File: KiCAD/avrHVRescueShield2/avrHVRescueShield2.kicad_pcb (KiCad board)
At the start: 2 copper layers, 69.8 x 54.6 mm, 24 parts, among them Q1 MUN5311DW1T1G, SW1 SW_Push, U1 ATmega328P-PU, U2 ATtiny85-20PU, U3 ATtiny2313-20PU, U4 MC34063AP

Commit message: error in schematics
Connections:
- U1 pad 1: unconnected-(U1-Pad1) -> ~{RESET}
- U1 pad 21: ~{RESET} -> unconnected-(U1-Pad21)
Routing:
- net GND: track 203.6 -> 390.5 mm
- net ~{RESET}: track 93.3 -> 0.00 mm
- net RDY: track 54.4 -> 0.00 mm
- net DATA6: track 39.2 -> 0.00 mm

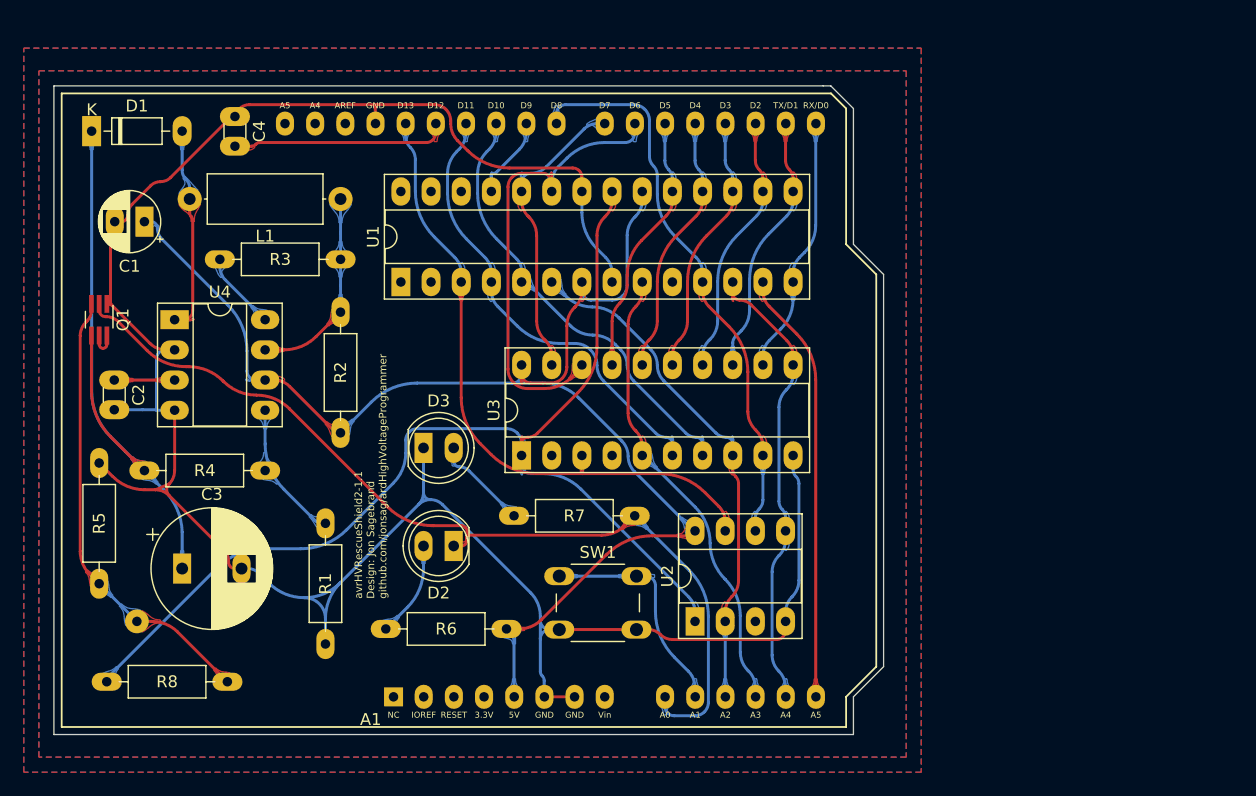
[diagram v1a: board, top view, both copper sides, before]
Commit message: new PCB
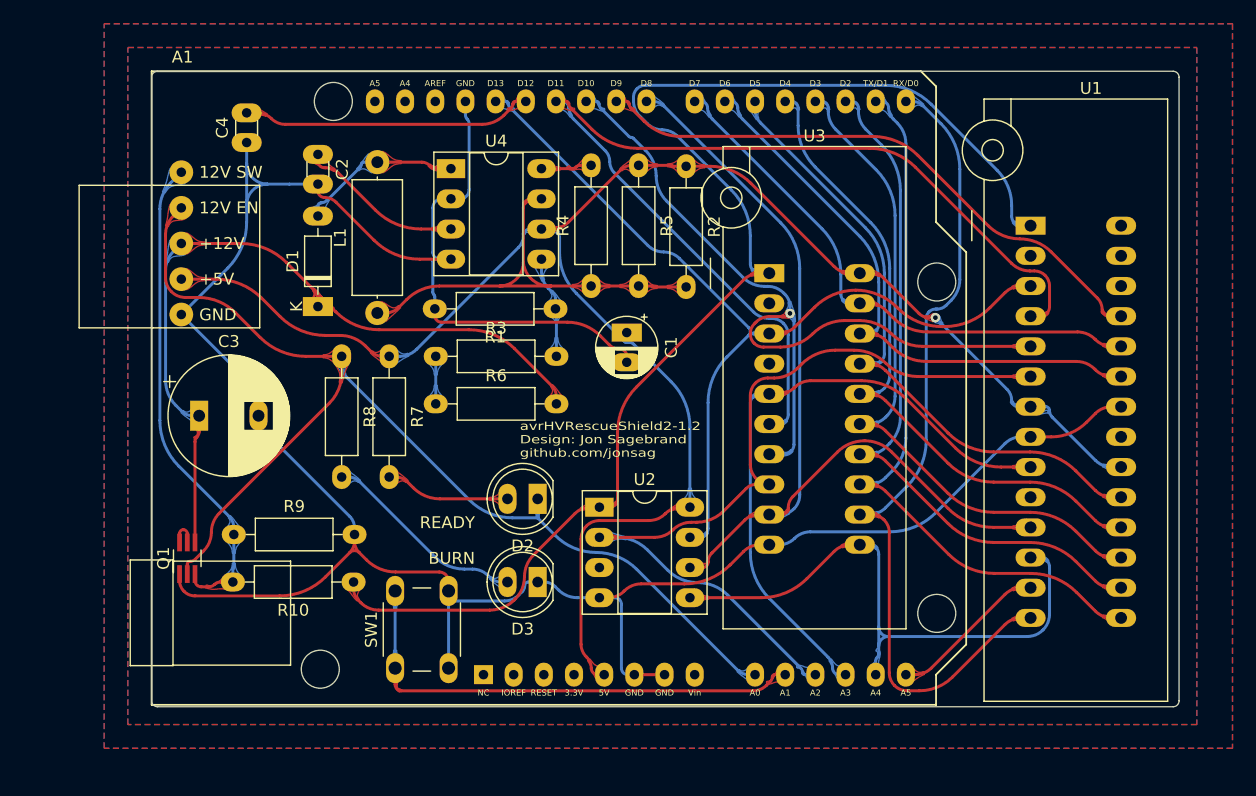
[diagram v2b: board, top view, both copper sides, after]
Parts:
- added R10: 100R, My_Misc:R_Axial_DIN0207_L6.3mm_D2.5mm_P10.16mm_Horizontal_large, F.Cu at (130.0, 104.0)
- added R9: 1k, My_Misc:R_Axial_DIN0207_L6.3mm_D2.5mm_P10.16mm_Horizontal_large, F.Cu at (119.9, 100.0)
- added TP2: 12V EN, My_Misc:Single_solder_pad, F.Cu at (115.5, 72.5)
- added TP3: 12V SW, My_Misc:Single_solder_pad, F.Cu at (115.5, 69.5)
- added TP4: +5V, My_Misc:Single_solder_pad, F.Cu at (115.5, 78.5)
- added TP5: GND, My_Misc:Single_solder_pad, F.Cu at (115.5, 81.5)
- R1, R7: footprint My_Misc:R_Axial_DIN0207_L6.3mm_D2.5mm_P10.16mm_Horizontal_larger_pads -> My_Misc:R_Axial_DIN0207_L6.3mm_D2.5mm_P10.16mm_Horizontal_large
- R2: value 0.5R -> 1R; footprint My_Misc:R_Axial_DIN0207_L6.3mm_D2.5mm_P10.16mm_Horizontal_larger_pads -> My_Misc:R_Axial_DIN0207_L6.3mm_D2.5mm_P10.16mm_Horizontal_large
- R3: value 180R -> 12k; footprint My_Misc:R_Axial_DIN0207_L6.3mm_D2.5mm_P10.16mm_Horizontal_larger_pads -> My_Misc:R_Axial_DIN0207_L6.3mm_D2.5mm_P10.16mm_Horizontal_large
- R4: value 13k -> 180R; footprint My_Misc:R_Axial_DIN0207_L6.3mm_D2.5mm_P10.16mm_Horizontal_larger_pads -> My_Misc:R_Axial_DIN0207_L6.3mm_D2.5mm_P10.16mm_Horizontal_large
- R5: value 1k -> 1R; footprint My_Misc:R_Axial_DIN0207_L6.3mm_D2.5mm_P10.16mm_Horizontal_larger_pads -> My_Misc:R_Axial_DIN0207_L6.3mm_D2.5mm_P10.16mm_Horizontal_large
- R6: value 330R -> 1k; footprint My_Misc:R_Axial_DIN0207_L6.3mm_D2.5mm_P10.16mm_Horizontal_larger_pads -> My_Misc:R_Axial_DIN0207_L6.3mm_D2.5mm_P10.16mm_Horizontal_large
- R8: value 100R -> 330R; footprint My_Misc:R_Axial_DIN0207_L6.3mm_D2.5mm_P10.16mm_Horizontal_larger_pads -> My_Misc:R_Axial_DIN0207_L6.3mm_D2.5mm_P10.16mm_Horizontal_large
- TP1: value TestPoint -> +12V
- U1: footprint Package_DIP:DIP-28_W7.62mm_Socket_LongPads -> My_Misc:ZIF_DIP_Socket-28_W6.9_W7.62_W7.62_W12.7_W13.5_large
- U3: footprint Package_DIP:DIP-20_W7.62mm_Socket_LongPads -> My_Misc:ZIF_DIP_Socket-20_W4.3_W5.08_W7.62_W10.16_W10.9_3M_220-3342-00-0602J_large
- moved R5 57.5 mm to (154.0, 68.9), turned to -90 degrees
- moved A1 56.1 mm to (113.0, 61.0)
- moved U1 53.2 mm to (187.0, 74.0), turned to 0 degrees
- moved C1 41.7 mm to (153.0, 83.0), turned to -90 degrees
- moved R4 40.7 mm to (150.0, 79.1), turned to 90 degrees
- moved R2 36.7 mm to (158.0, 69.0), turned to -90 degrees
- moved R8 33.8 mm to (129.0, 85.0), turned to -90 degrees
- moved TP1 32.0 mm to (115.5, 75.5), turned to 90 degrees
- moved U4 26.5 mm to (138.2, 69.2)
- moved R1 26.5 mm to (147.0, 81.0), turned to 180 degrees
- moved U3 25.9 mm to (165.0, 78.0), turned to 0 degrees
- moved C2 25.6 mm to (127.0, 68.0)
- moved R7 24.6 mm to (133.0, 85.0), turned to -90 degrees
- moved D1 24.1 mm to (127.0, 80.8), turned to 90 degrees
- moved Q1 21.4 mm to (116.0, 102.0), turned to 90 degrees
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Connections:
- R3 pad 1: Net-(L1-Pad1) -> Net-(R3-Pad1)
- R3 pad 2: Net-(R3-Pad2) -> Net-(R1-Pad1)
- R4 pad 1: +12V -> Net-(L1-Pad1)
- R4 pad 2: Net-(R1-Pad1) -> Net-(R4-Pad2)
- R5 pad 1: 12V_SW -> +5V
- R5 pad 2: GND -> Net-(L1-Pad1)
- R6 pad 1: +5V -> Net-(R3-Pad1)
- R6 pad 2: Net-(D2-Pad2) -> +12V
- R7 pad 1: 12V_EN -> +5V
- R7 pad 2: Net-(D3-Pad2) -> Net-(D2-Pad2)
- R8 pad 1: ~{RESET} -> 12V_EN
- R8 pad 2: 12V_SW -> Net-(D3-Pad2)
- TP1 pad 1: 12V_SW -> +12V
- U4 pad 8: Net-(R3-Pad2) -> Net-(R4-Pad2)
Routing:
- net GND: track 390.5 -> 216.4 mm
- net ~{RESET}: track 0.00 -> 113.8 mm
- net RDY: track 0.00 -> 76.2 mm
- net ~{OE}: track 38.0 -> 88.8 mm
- net DATA0: track 21.7 -> 71.5 mm
- net DATA6: track 0.00 -> 49.2 mm
- net BS2: track 6.93 -> 49.6 mm
- net DATA1: track 22.1 -> 61.7 mm
- net DATA2: track 22.0 -> 59.7 mm
- net DATA3: track 22.0 -> 57.9 mm
- net DATA4: track 22.0 -> 55.9 mm
- net +5V: track 118.2 -> 150.9 mm, vias 0 -> 1
- net DATA5: track 22.1 -> 53.9 mm
- net ~{WR}: track 37.9 -> 69.4 mm, vias 0 -> 1
- net XA0: track 47.5 -> 78.3 mm
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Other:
- board size 69.8 x 54.6 mm -> 86.5 x 53.5 mm
- board text added: "${TITLE}-${REVISION} Design: Jon Sagebrand github.com/jonsag"
- board text added: "+12V"
- board text added: "+5V"
- board text added: "12V EN"
- board text added: "12V SW"
- board text added: "BURN"
- board text added: "GND"
- board text added: "READY"
- board text removed: "${TITLE}-${REVISION} Design: Jon Sagebrand github.com/jonsag/ardHighVoltageProgrammer"
